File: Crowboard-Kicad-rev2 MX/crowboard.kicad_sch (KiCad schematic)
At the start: 78 parts, among them U1 Pico

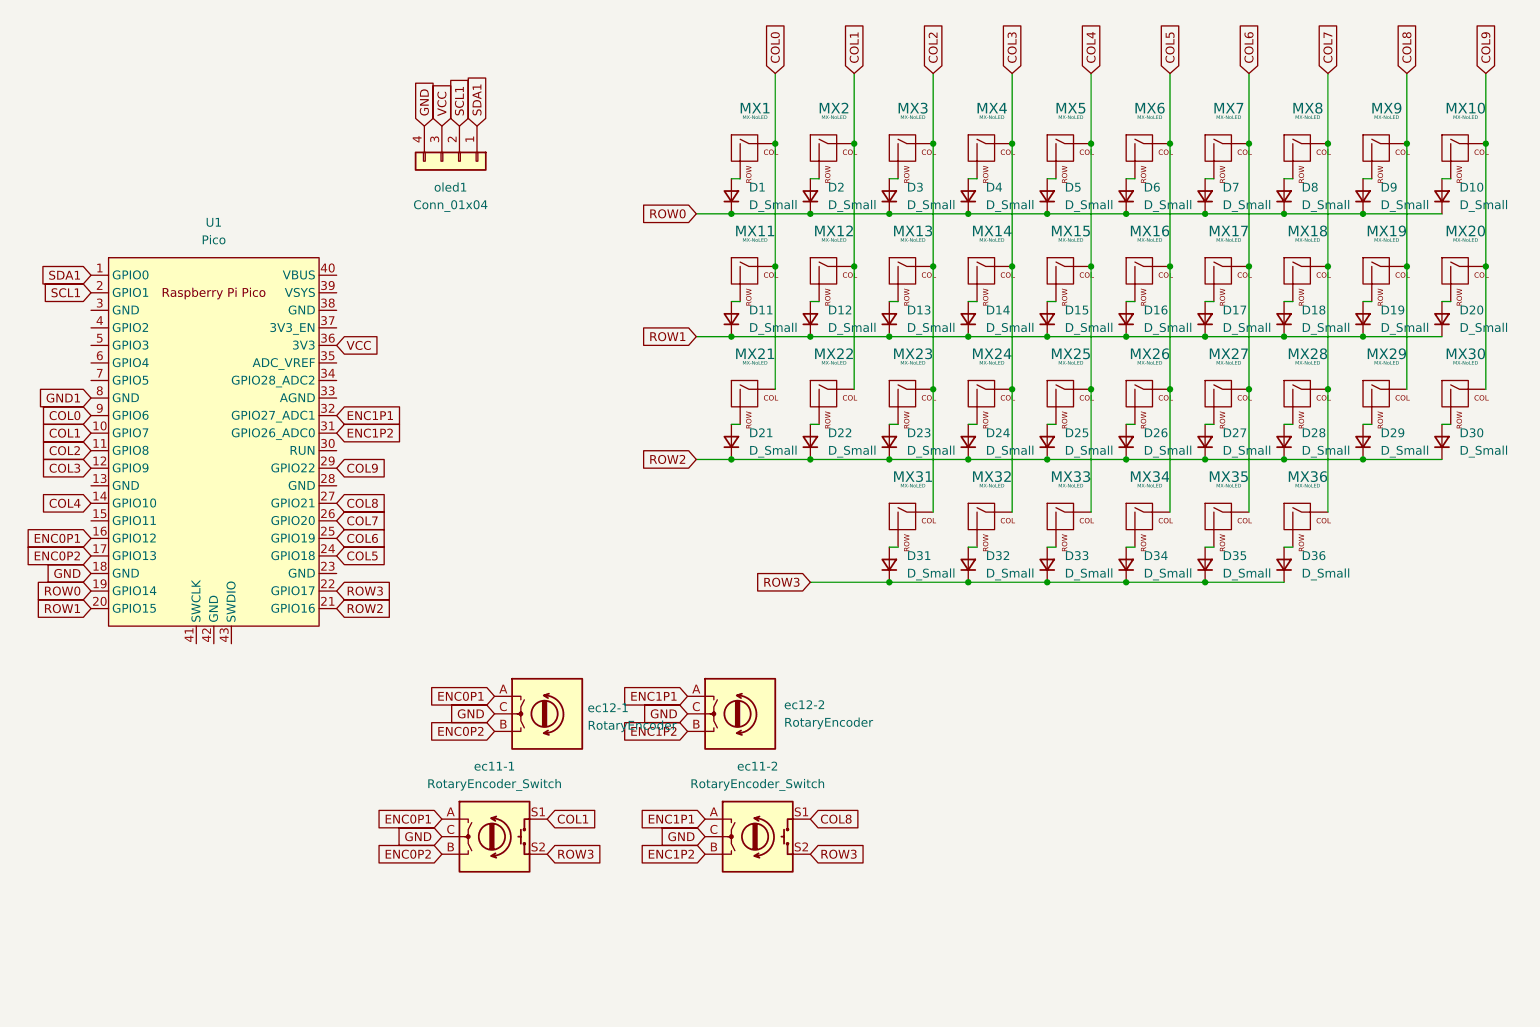
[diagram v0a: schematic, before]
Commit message: 4 encoders
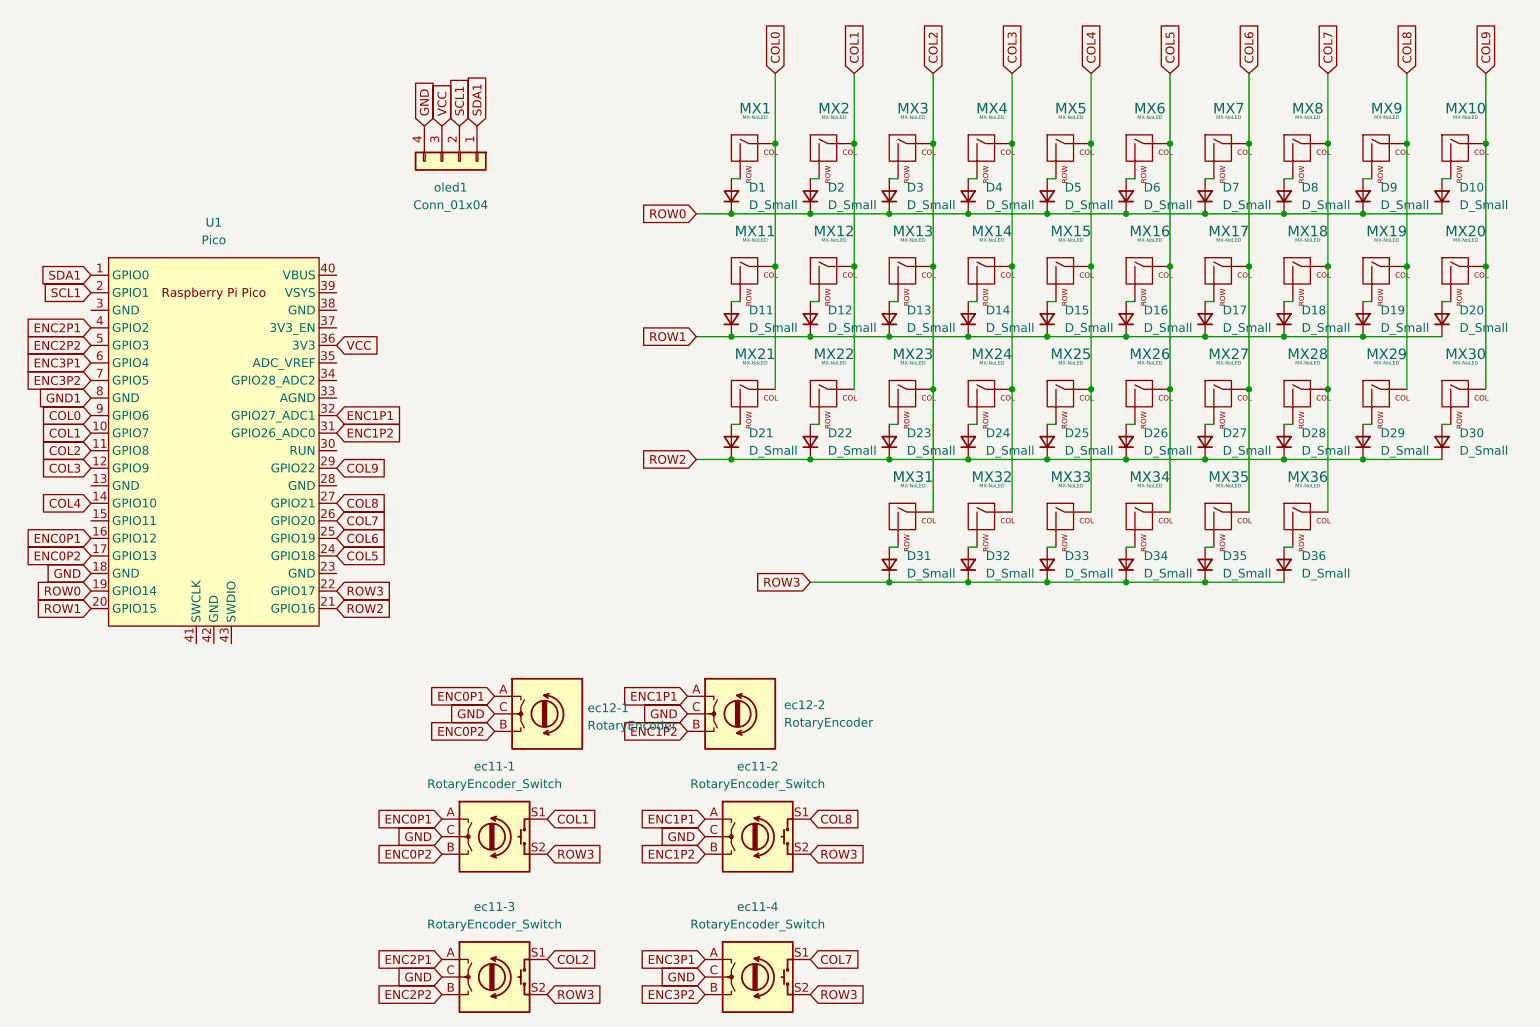
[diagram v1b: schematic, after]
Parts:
- added ec11-3, ec11-4: RotaryEncoder_Switch, Rotary_Encoder:RotaryEncoder_Alps_EC11E-Switch_Vertical_H20mm, symbol Device:RotaryEncoder_Switch
- MX1, MX10, MX11, MX12, MX13, MX14, MX15, MX16, MX17, MX18, MX19, MX2, MX20, MX21, MX22, MX23, MX24, MX25, MX26, MX27, MX28, MX29, MX3, MX30, MX31, MX32, MX33, MX34, MX35, MX36, MX4, MX5, MX6, MX7, MX8, MX9: footprint (none) -> MX_Only:MXOnly-1U-NoLED
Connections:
- net COL2: now also ec11-3.S1
- net COL7: now also ec11-4.S1
- net GND: now also ec11-3.C, ec11-4.C
- net ROW3: now also ec11-3.S2, ec11-4.S2
- net ENC2P1: now reaches U1.4 (GPIO2)
- net ENC2P1: now also ec11-3.A
- net ENC2P2: now reaches U1.5 (GPIO3)
- net ENC2P2: now also ec11-3.B
- net ENC3P1: now reaches U1.6 (GPIO4)
- net ENC3P1: now also ec11-4.A
- net ENC3P2: now reaches U1.7 (GPIO5)
- net ENC3P2: now also ec11-4.B
